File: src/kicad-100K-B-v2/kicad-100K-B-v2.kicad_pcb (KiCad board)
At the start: 2 copper layers, 35.6 x 48.3 mm, 29 parts, among them P1 In, P2 Out, P3 Power, U1 TL072

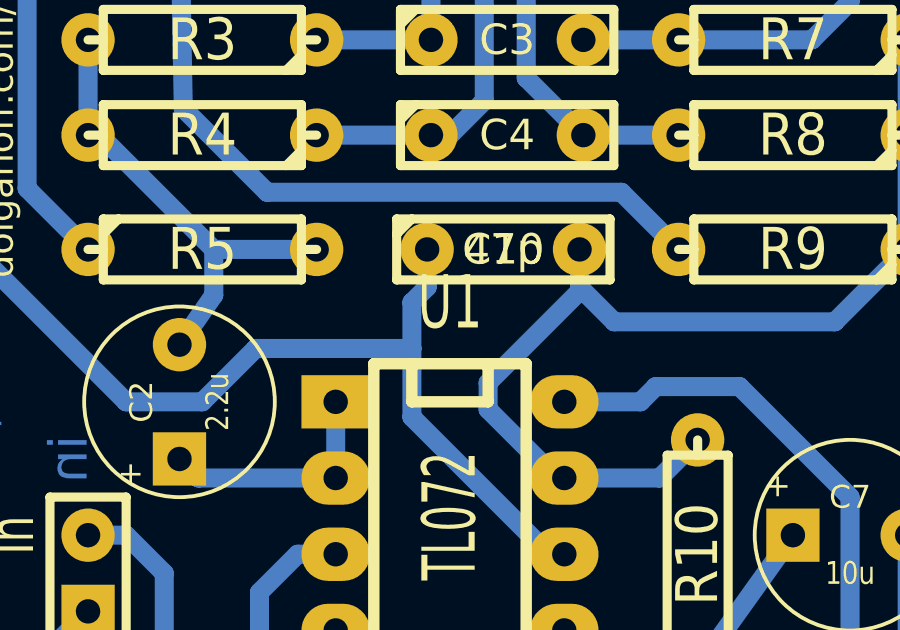
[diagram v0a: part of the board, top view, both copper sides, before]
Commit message: changes in bass version
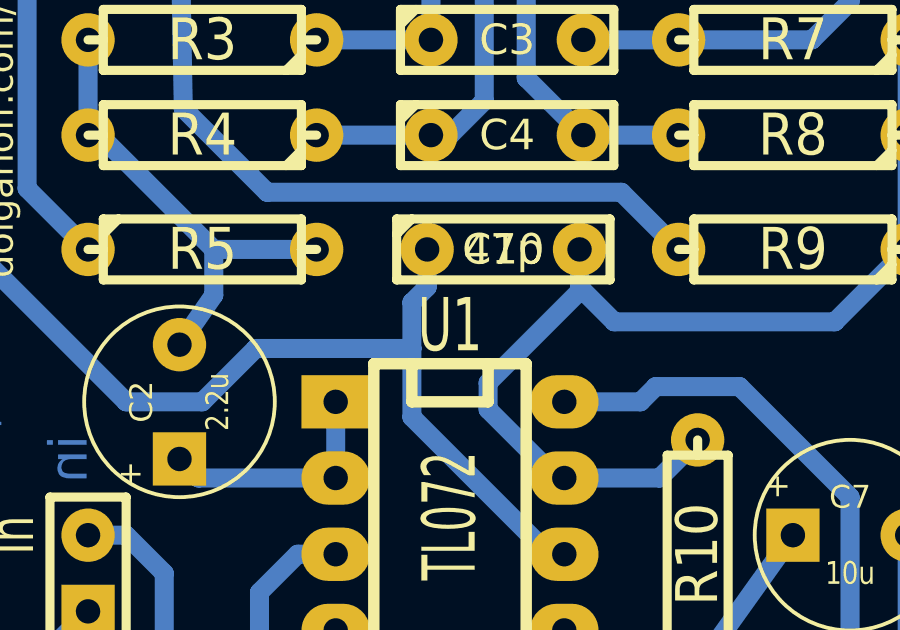
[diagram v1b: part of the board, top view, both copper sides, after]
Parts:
- R10: value 500 -> 470
- R2: value 5Meg -> 4.7 Meg
